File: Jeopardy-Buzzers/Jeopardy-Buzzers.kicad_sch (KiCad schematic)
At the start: 13 parts, among them J1 USB_C_Receptacle, U1 CH32V003FxUx, U2 CH340N, U3 NRF24L01_Breakout, U4 TPD2EUSB30, U5 AMS1117-3.3

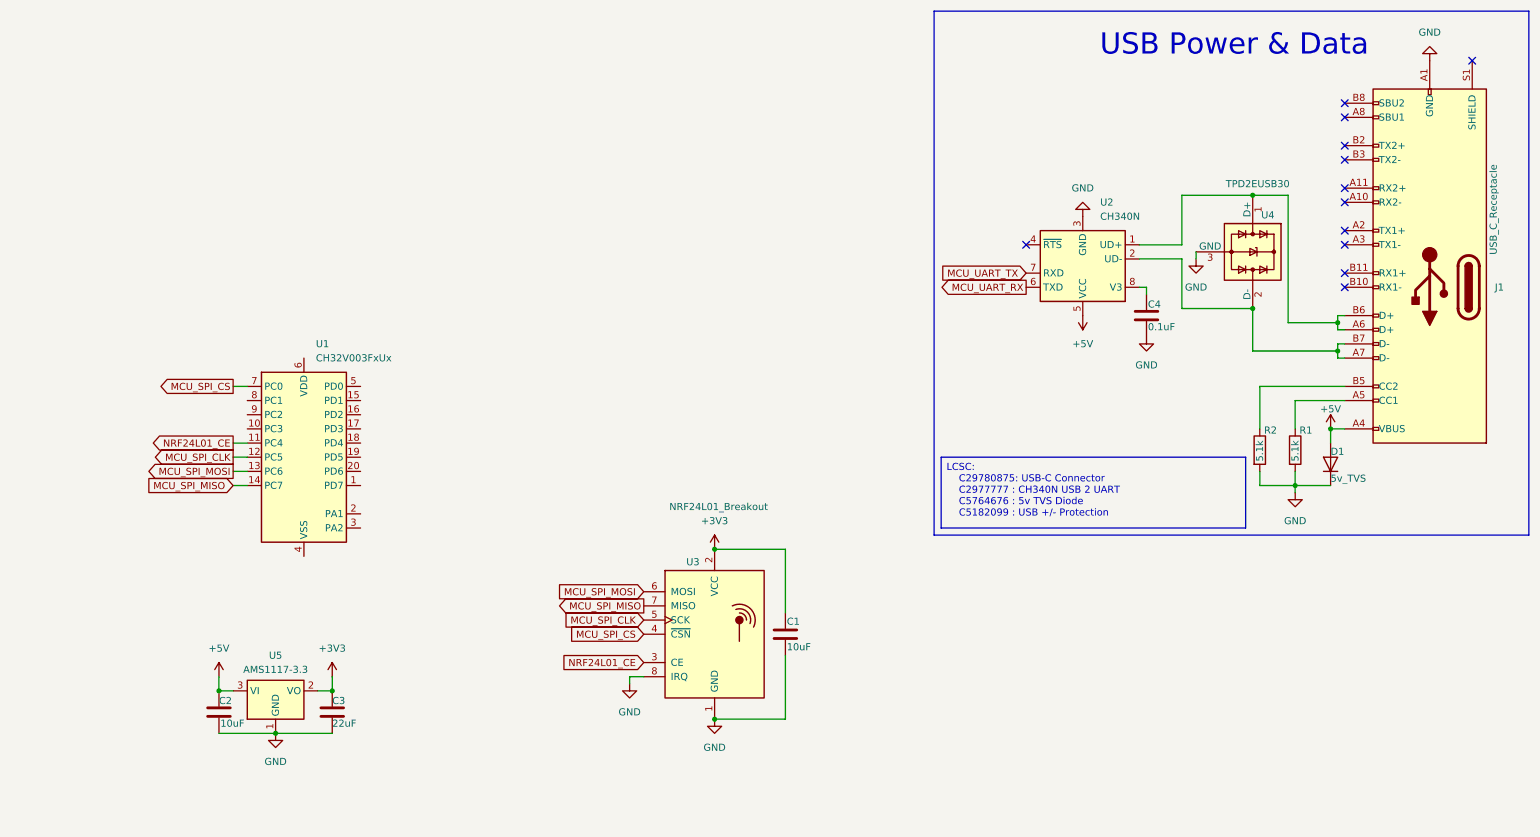
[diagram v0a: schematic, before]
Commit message: Cleaned up the NRF24L01 & LDO
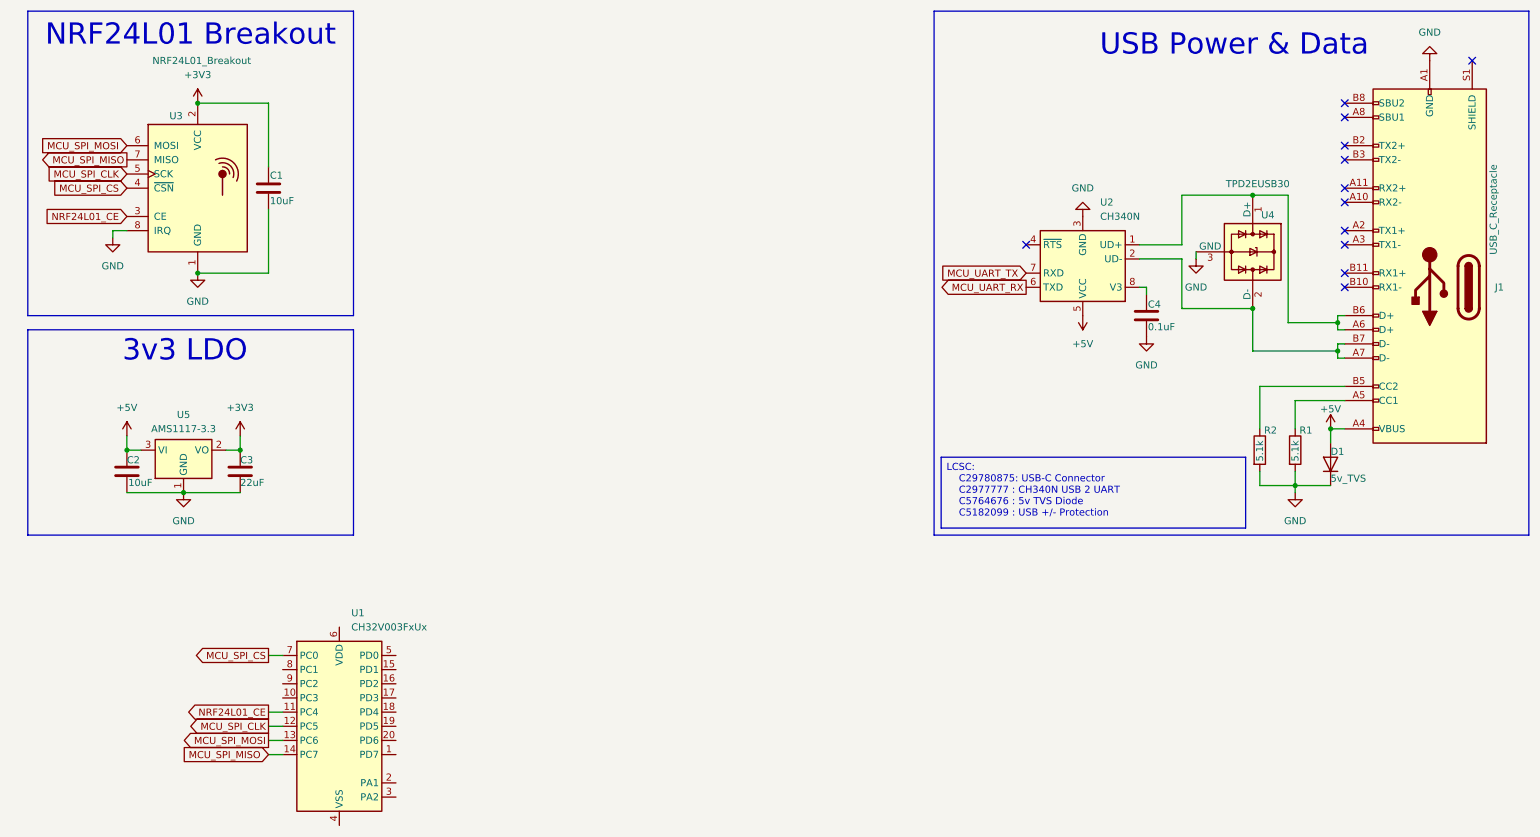
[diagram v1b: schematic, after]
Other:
- note added: "3v3 LDO"
- note added: "NRF24L01 Breakout"
- moved on the sheet: C1, C2, C3, U1, U3, U5
